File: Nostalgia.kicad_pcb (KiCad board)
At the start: 2 copper layers, 70 x 102 mm, 46 parts, among them J10 490107670612, J20 USB-C6, K85 Val, U30 1117-3.3, U40 ESP32-S3-WROOM-1-N16R8

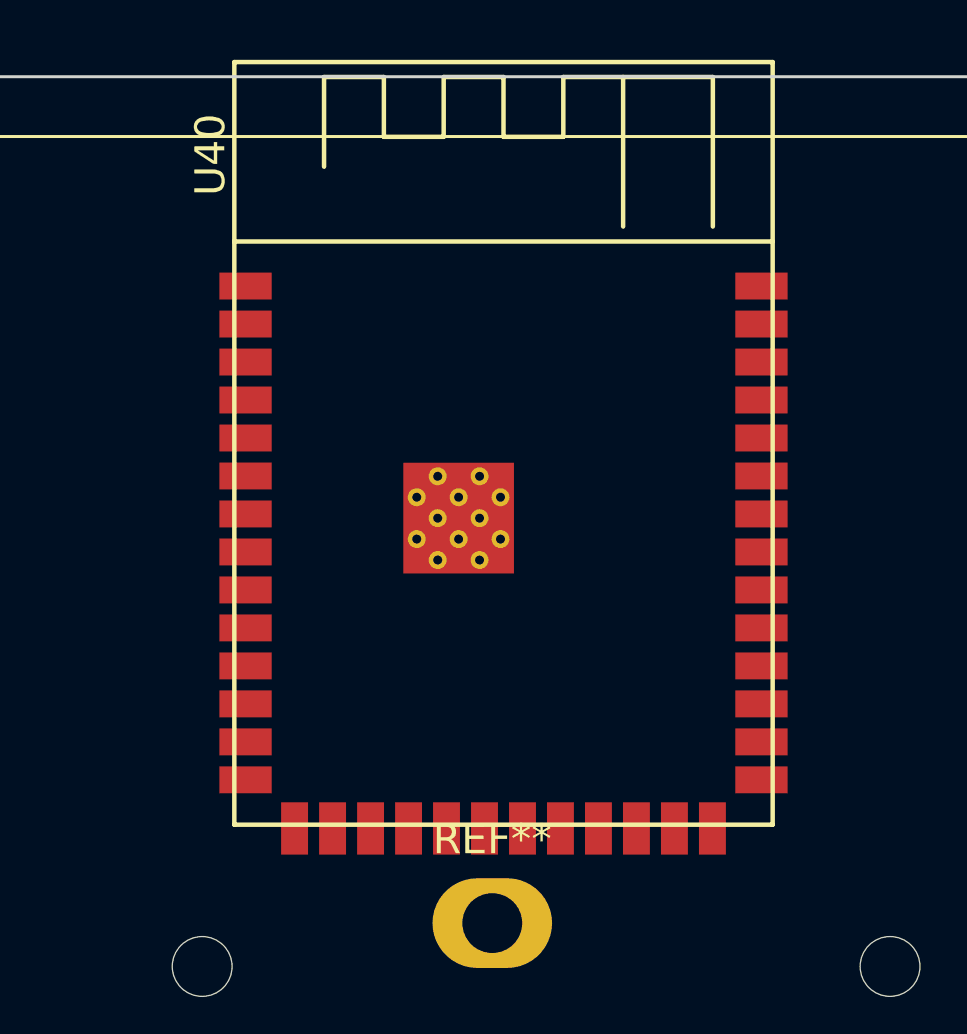
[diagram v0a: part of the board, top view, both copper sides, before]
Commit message: WIP
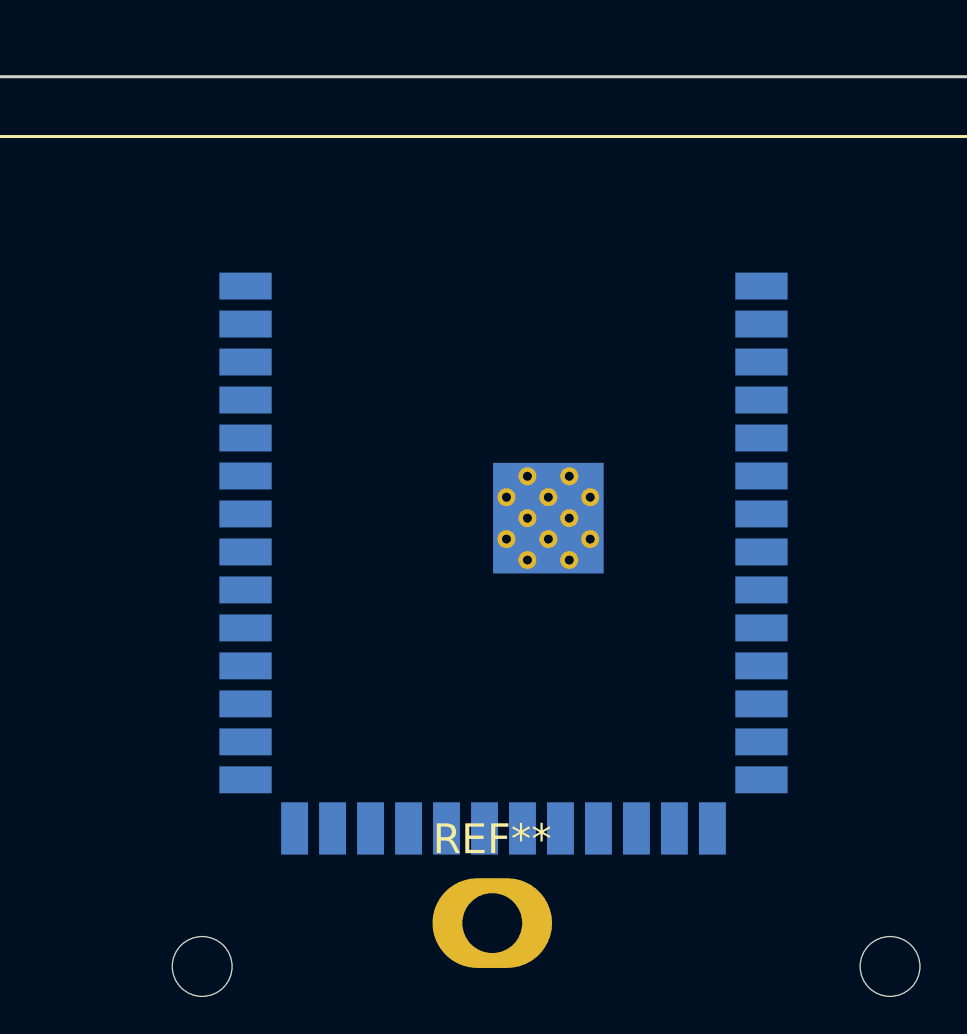
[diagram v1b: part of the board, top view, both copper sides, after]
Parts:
- U40: moved to B.Cu
- turned U40 to 180 degrees
